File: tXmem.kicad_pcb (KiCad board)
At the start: 2 copper layers, 39 x 65 mm, 37 parts, among them U1 74LCX125, U10 SPIMEMORY, U11 SPIMEMORY, U12 SPIMEMORY, U13 SPIMEMORY, U14 SPIMEMORY, U15 SPIMEMORY, U16 SPIMEMORY, U17 SPIMEMORY, U18 SPIMEMORY, U19 SPIMEMORY, U2 74LCX138, U3 74LCX138, U4 SPIMEMORY, U5 SPIMEMORY, U6 SPIMEMORY, U7 SPIMEMORY, U8 SPIMEMORY, U9 SPIMEMORY

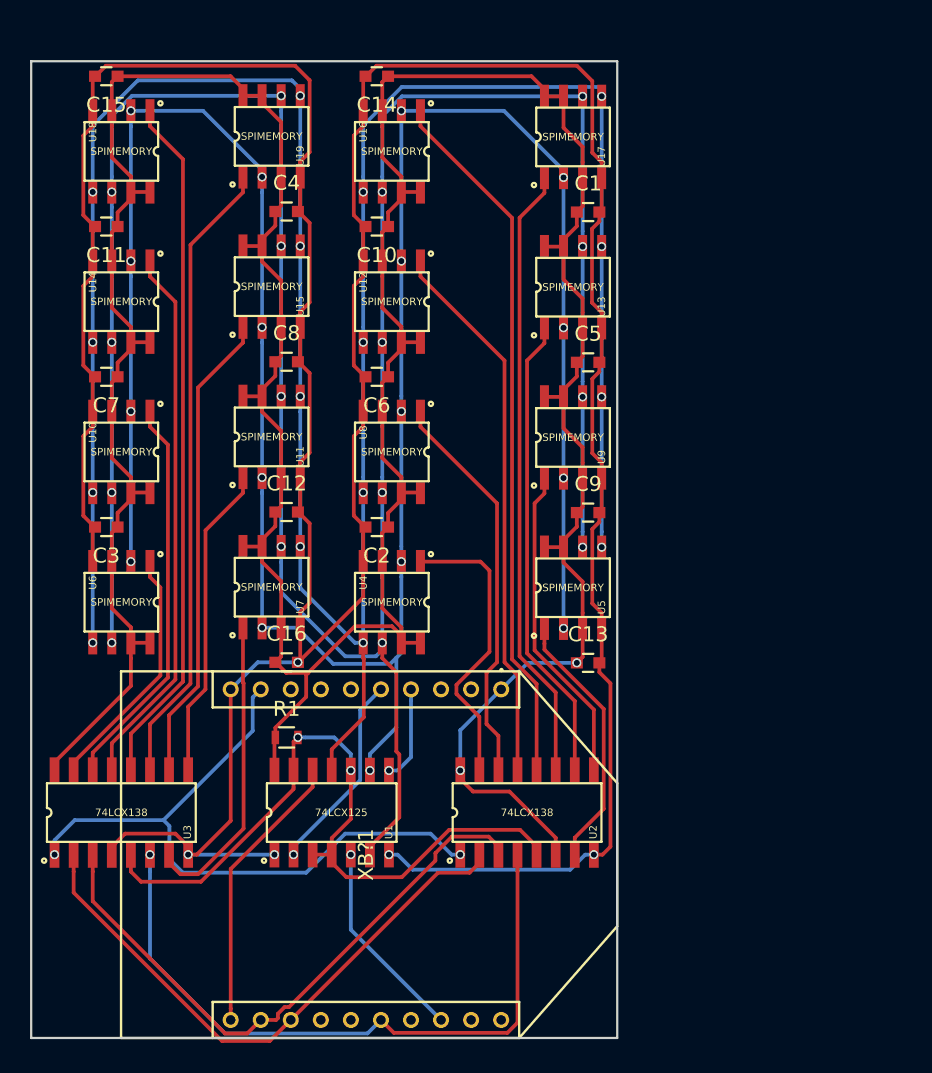
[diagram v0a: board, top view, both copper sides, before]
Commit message: work in progress
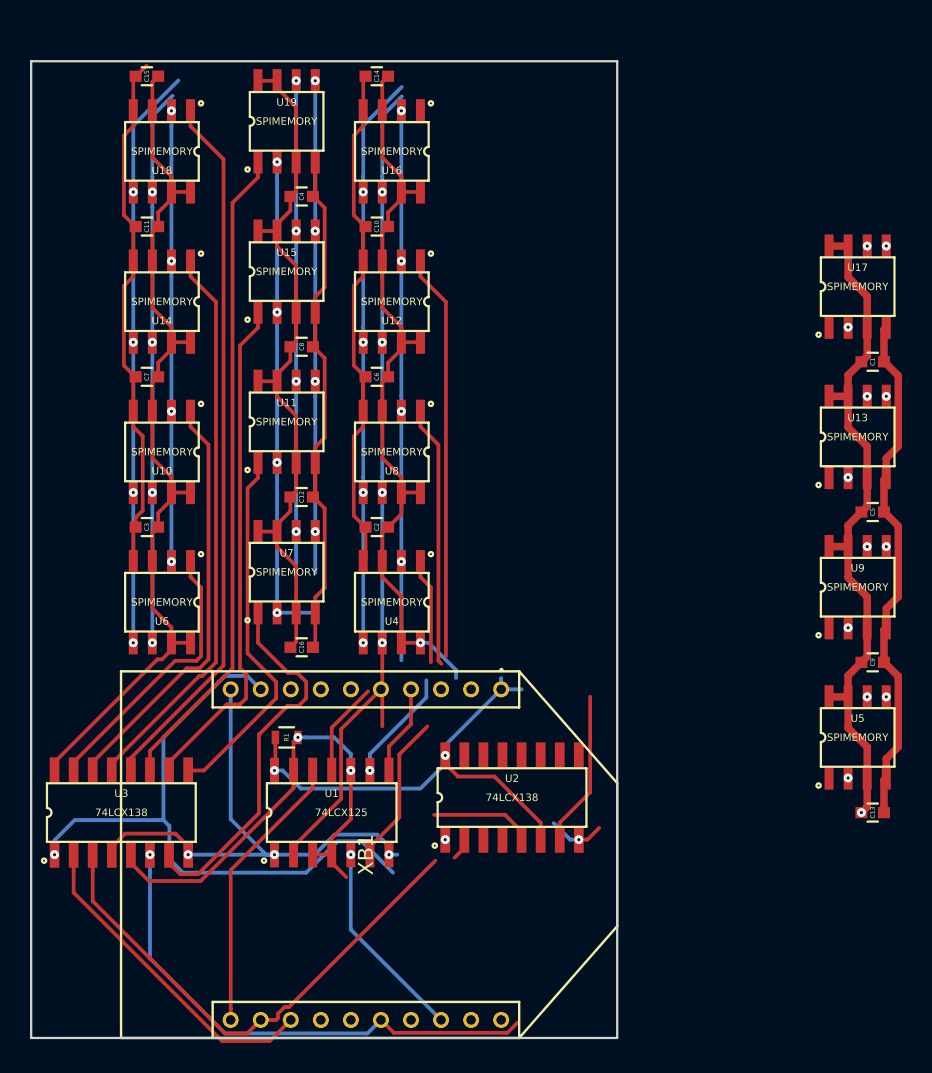
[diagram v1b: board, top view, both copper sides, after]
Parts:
- removed XB?1: XBEE, tXmem:XBee
- added XB1: XBEE, tXmem:XBee, F.Cu at (102.3, 112.8)
- moved C1 21.4 mm to (136.0, 80.0)
- moved C13 21.4 mm to (136.0, 110.0)
- moved C5 21.4 mm to (136.0, 90.0)
- moved C9 21.4 mm to (136.0, 100.0)
- moved U13 21.4 mm to (135.0, 85.0)
- moved U17 21.4 mm to (135.0, 75.0)
- moved U5 21.4 mm to (135.0, 105.0)
- moved U9 21.4 mm to (135.0, 95.0)
- moved C11 2.70 mm to (87.7, 71.0)
- moved C15 2.70 mm to (87.7, 61.0)
- moved C3 2.70 mm to (87.7, 91.0)
- moved C7 2.70 mm to (87.7, 81.0)
- moved U10 2.70 mm to (88.7, 86.0)
- moved U14 2.70 mm to (88.7, 76.0)
- moved U18 2.70 mm to (88.7, 66.0)
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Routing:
- net GND: track 248.3 -> 178.2 mm, vias 5 -> 4
- net /SI: track 179.9 -> 115.8 mm
- net /SO: track 168.6 -> 106.5 mm
- net /SCK: track 183.4 -> 122.6 mm
- net /D12: track 47.1 -> 0.00 mm
- net /D11: track 41.1 -> 0.00 mm
- net /D10: track 31.3 -> 0.00 mm
- net /D9: track 21.4 -> 0.00 mm
- net VCC: track 257.6 -> 237.8 mm, vias 2 -> 4
- net /A1: track 39.1 -> 23.1 mm
- net /D15: track 19.7 -> 6.99 mm
- net /A3: track 45.6 -> 34.4 mm
- net /D14: track 26.6 -> 17.4 mm
- net /D13: track 36.6 -> 27.6 mm
- net /~CS: track 47.7 -> 39.1 mm
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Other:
- net class Default: via_drill 0.4 -> 0.2
- rule via_min_drill: 0.3 -> 0.18

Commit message: dwarfing!
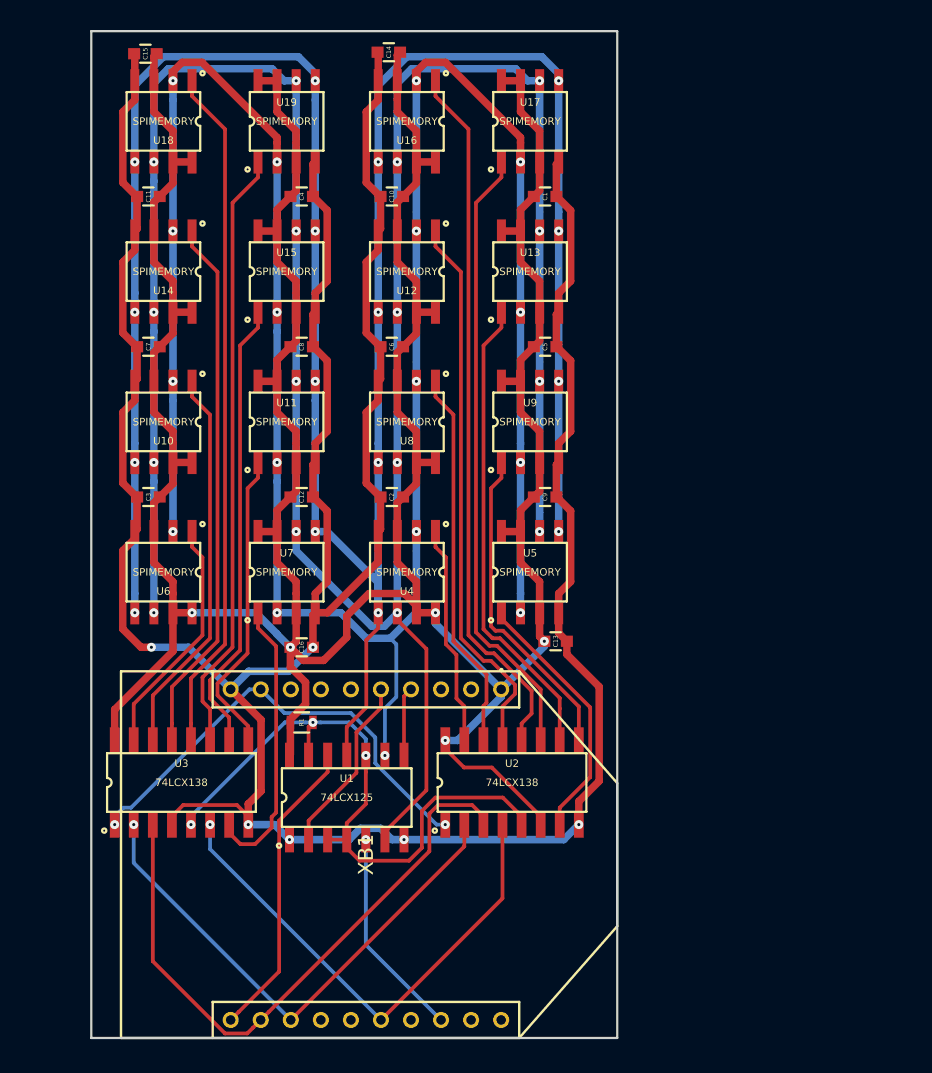
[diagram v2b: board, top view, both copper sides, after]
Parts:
- moved C1 24.4 mm to (114.2, 69.0)
- moved C5 24.4 mm to (114.2, 79.0)
- moved C9 24.4 mm to (114.2, 89.0)
- moved U13 24.4 mm to (113.2, 74.0)
- moved U17 24.4 mm to (113.2, 64.0)
- moved U5 24.4 mm to (113.2, 94.0)
- moved U9 24.4 mm to (113.2, 84.0)
- moved C13 24.0 mm to (114.9, 98.6)
- moved U3 4.47 mm to (90.0, 108.0)
- moved C10 2.24 mm to (104.0, 69.0)
- moved C2 2.24 mm to (104.0, 89.0)
- moved C6 2.24 mm to (104.0, 79.0)
- moved U12 2.24 mm to (105.0, 74.0)
- moved U16 2.24 mm to (105.0, 64.0)
- moved U4 2.24 mm to (105.0, 94.0)
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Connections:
- net Net-(U1-Pad2) renamed /~E
- XB1 pad 15: (no net) -> Net-(XB1-Pad15)
- XB1 pad 17: (no net) -> Net-(XB1-Pad17)
- XB1 pad 19: (no net) -> Net-(XB1-Pad19)
- XB1 pad 2: (no net) -> Net-(XB1-Pad2)
- XB1 pad 20: (no net) -> Net-(XB1-Pad20)
- XB1 pad 3: (no net) -> Net-(XB1-Pad3)
- XB1 pad 7: (no net) -> Net-(XB1-Pad7)
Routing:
- net /SO: track 106.5 -> 167.3 mm
- net /SI: track 115.8 -> 175.6 mm
- net /SCK: track 122.6 -> 178.4 mm
- net /D12: track 0.00 -> 47.1 mm
- net GND: track 178.2 -> 223.2 mm, vias 4 -> 6
- net /D11: track 0.00 -> 41.3 mm
- net /D10: track 0.00 -> 31.4 mm
- net /D9: track 0.00 -> 21.5 mm
- net VCC: track 237.8 -> 250.8 mm, vias 4 -> 5
- net /A1: track 23.1 -> 35.1 mm, vias 0 -> 1
- net /A0: track 42.6 -> 30.8 mm
- net /D13: track 27.6 -> 36.7 mm
- net /D14: track 17.4 -> 25.4 mm
- net /D15: track 6.99 -> 14.7 mm
- net /D8: track 10.4 -> 17.4 mm
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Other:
- board size 39 x 65 mm -> 35 x 67 mm
